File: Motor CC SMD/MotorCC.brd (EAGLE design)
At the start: 47 x 58.1 mm, 11 parts

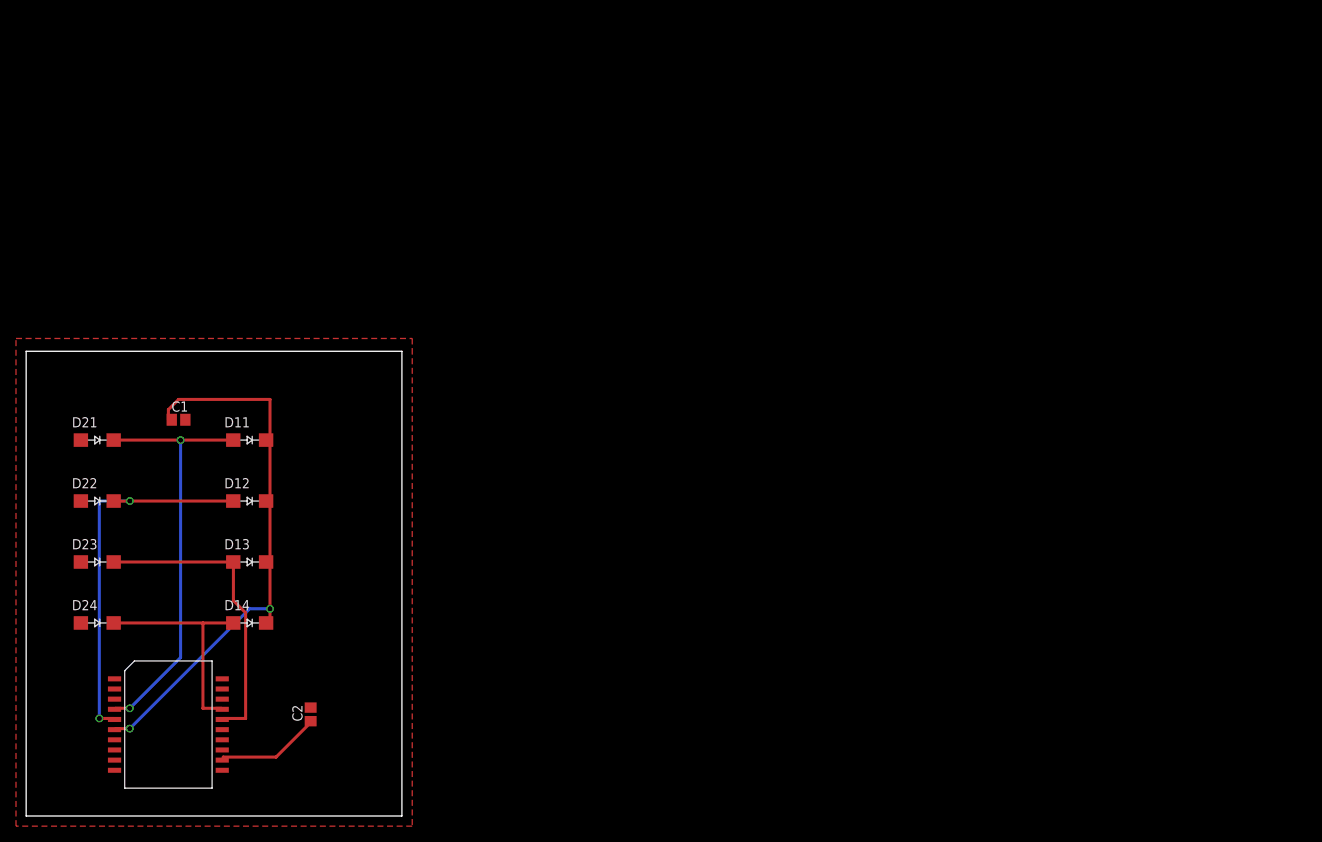
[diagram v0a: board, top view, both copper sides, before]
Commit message: Motors DC finished :D
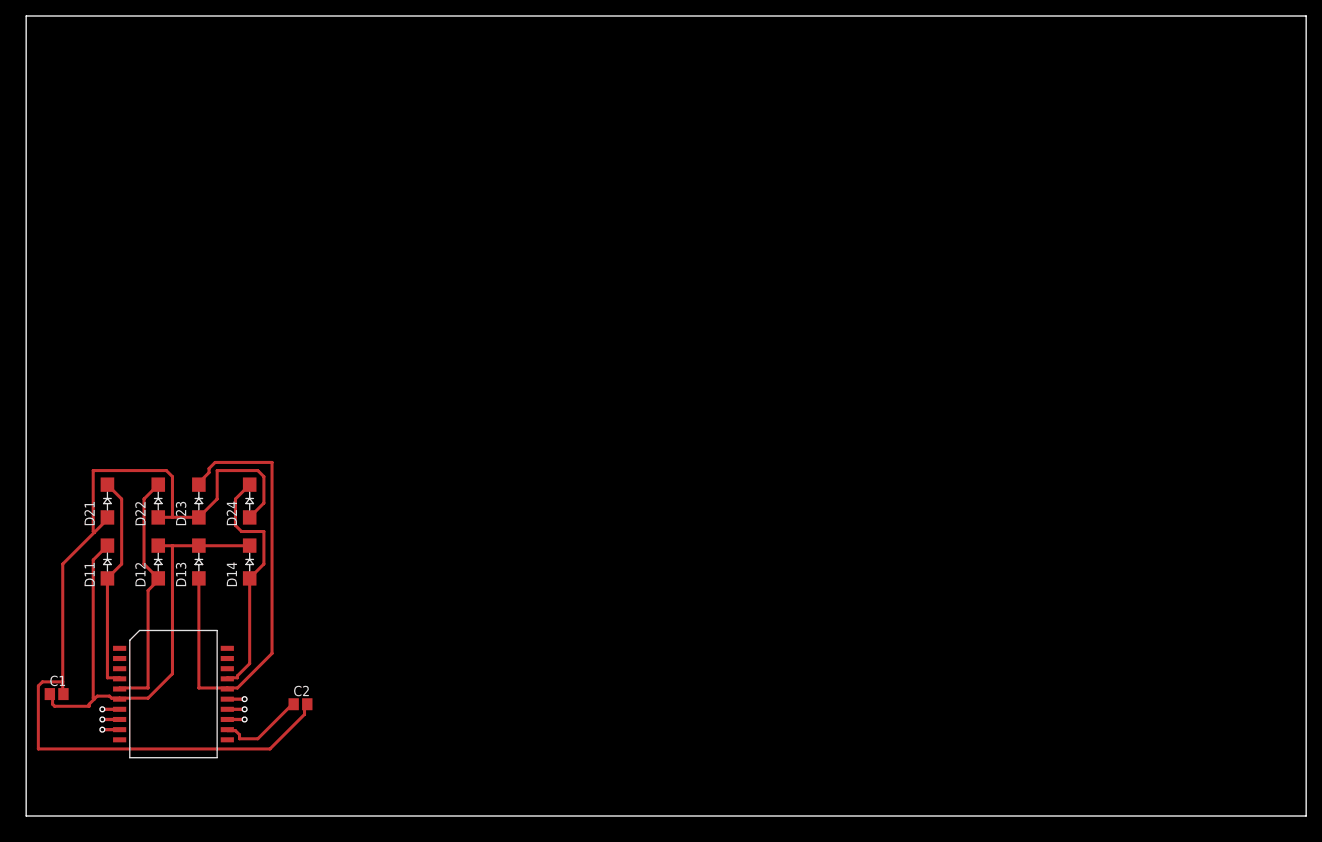
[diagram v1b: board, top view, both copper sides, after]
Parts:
- moved C1 37.5 mm to (3.81, 15.2)
- moved D24 24.4 mm to (27.9, 39.4), turned to 90 degrees
- moved D11 23.4 mm to (10.2, 31.8), turned to 90 degrees
- moved D23 14.8 mm to (21.6, 39.4), turned to 90 degrees
- moved D12 13.7 mm to (16.5, 31.8), turned to 90 degrees
- moved D21 7.73 mm to (10.2, 39.4), turned to 90 degrees
- moved D14 7.62 mm to (27.9, 31.8), turned to 90 degrees
- moved D22 7.62 mm to (16.5, 39.4), turned to 90 degrees
- moved D13 6.35 mm to (21.6, 31.8), turned to 90 degrees
- moved U$1 3.86 mm to (18.4, 15.2)
- moved C2 1.80 mm to (34.3, 14.0), turned to 0 degrees
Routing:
- net GND: track 0.00 -> 119.1 mm
- net N$1: track 53.1 -> 27.3 mm, vias 2 -> 0
- net N$3: track 38.1 -> 59.4 mm
- net N$2: track 47.9 -> 31.1 mm, vias 2 -> 0
- net VSS: track 70.5 -> 66.2 mm, vias 2 -> 0
- net N$4: track 28.1 -> 30.8 mm
- net VCC: track 13.3 -> 10.9 mm
- net N$7: track 0.00 -> 1.91 mm
- net N$6: track 0.00 -> 1.91 mm
- net N$5: track 0.00 -> 1.91 mm
- net N$9: track 0.00 -> 1.90 mm
- net N$8: track 0.00 -> 1.90 mm
- net N$10: track 0.00 -> 1.90 mm
- removed copper zone on layer 1, net GND
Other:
- board size 47 x 58.1 mm -> 160 x 100 mm
